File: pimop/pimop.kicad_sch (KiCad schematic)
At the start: 4 parts

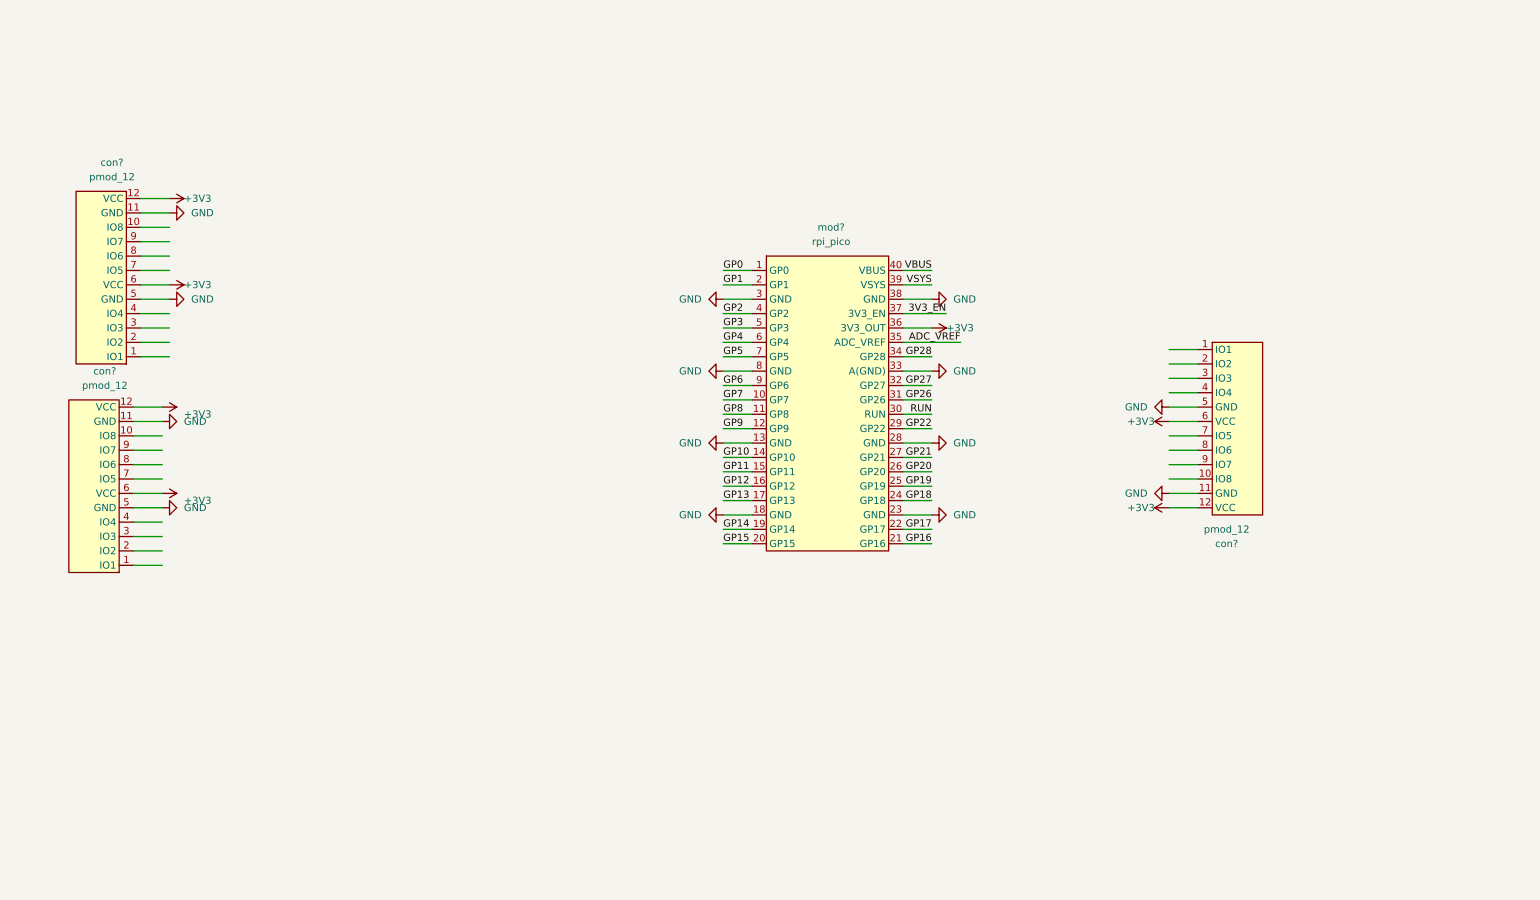
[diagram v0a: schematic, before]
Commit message: schema afgewerkt
schema afgewerkt
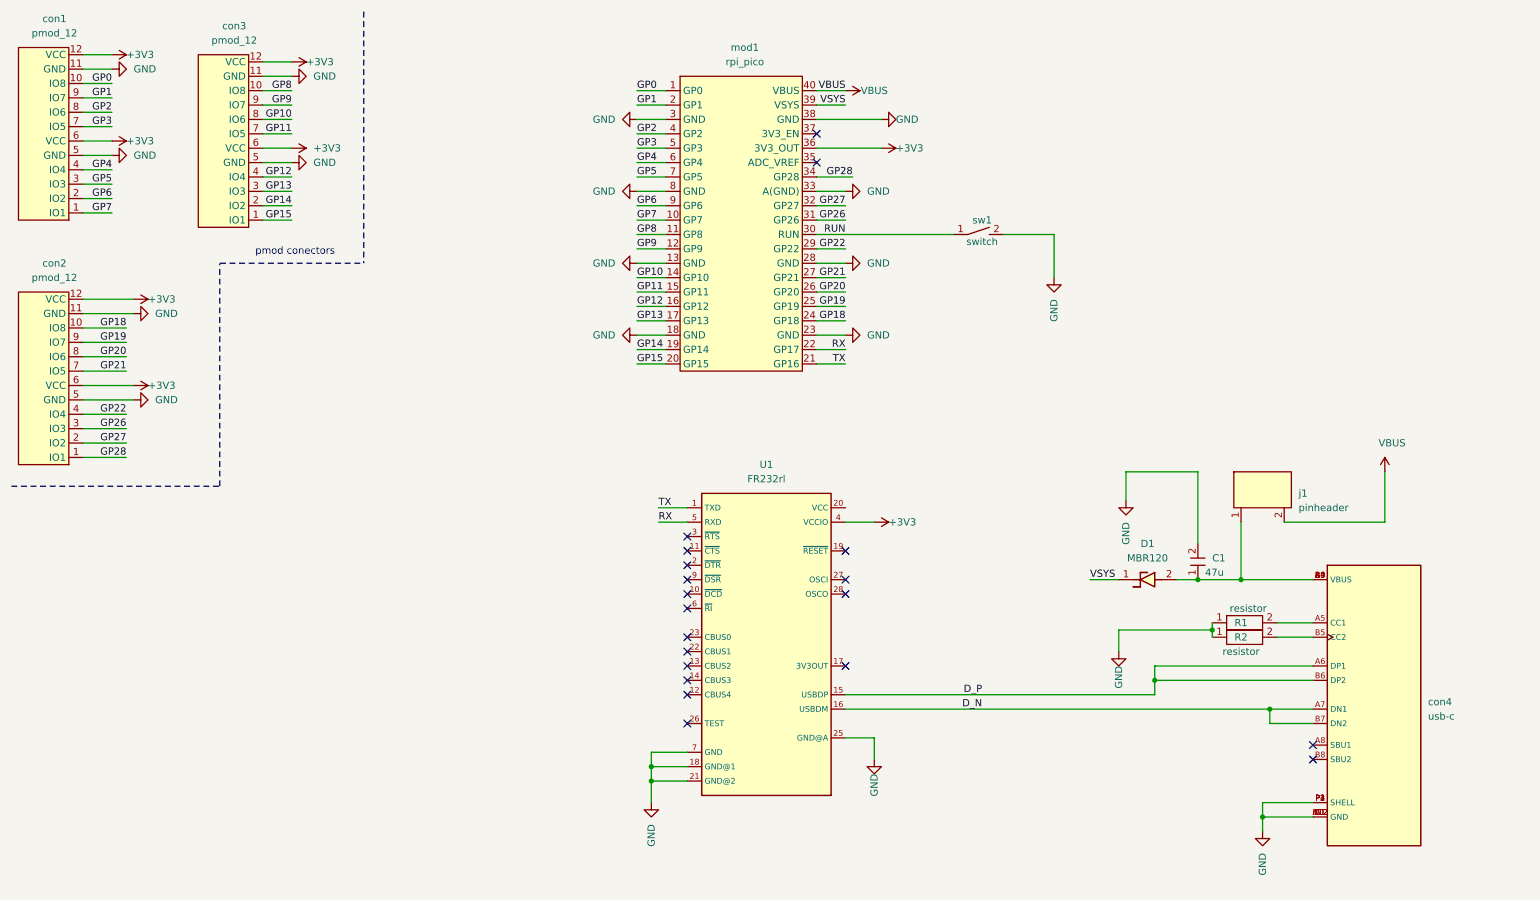
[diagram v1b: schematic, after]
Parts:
- added C1: 47u, vanalles:0603RL, symbol vanalles:capacitor
- added D1: MBR120, halfgeleiders:SOD123, symbol Halfgelijders:MBR120
- added R1, R2: resistor, vanalles:0603RL, symbol vanalles:resistor
- added U1: FR232rl, halfgeleiders:SSOP28-0.65-10.2X5.2MM, symbol Halfgelijders:FR232rl
- added con4: usb-c, connectors_user:GCT_USB4085-GF-A_REVA, symbol connectors:usb-c
- added j1: pinheader, connectors_user:heaer2pin, symbol vanalles:pinheader
- added sw1: switch, vanalles:Alps_SKRK, symbol vanalles:switch
- con1, con2, con3: renamed from con?; footprint (none) -> connectors_user:PMOD12
- mod1: renamed from mod?; footprint (none) -> Module:rpi pico
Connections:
- net +3V3: now also U1.4 (VCCIO)
- net GND: now also C1.2, R1.1, R2.1, U1.18 (GND@1), U1.21 (GND@2), U1.25 (GND@A), U1.7 (GND), con4.A1 (GND), con4.A12 (GND), con4.B1 (GND), con4.B12 (GND), con4.P1 (SHELL), con4.P2 (SHELL), con4.P3 (SHELL), con4.P4 (SHELL), sw1.2
- net GP0: now also con1.10 (IO8)
- net GP1: now also con1.9 (IO7)
- net GP10: now also con3.8 (IO6)
- net GP11: now also con3.7 (IO5)
- net GP12: now also con3.4 (IO4)
- net GP13: now also con3.3 (IO3)
- net GP14: now also con3.2 (IO2)
- net GP15: now also con3.1 (IO1)
- net GP18: now also con2.10 (IO8)
- net GP19: now also con2.9 (IO7)
- net GP2: now also con1.8 (IO6)
- net GP20: now also con2.8 (IO6)
- net GP21: now also con2.7 (IO5)
- net GP22: now also con2.4 (IO4)
- net GP26: now also con2.3 (IO3)
- net GP27: now also con2.2 (IO2)
- net GP28: now also con2.1 (IO1)
- net GP3: now also con1.7 (IO5)
- net GP4: now also con1.4 (IO4)
- net GP5: now also con1.3 (IO3)
- net GP6: now also con1.2 (IO2)
- net GP7: now also con1.1 (IO1)
- net GP8: now also con3.10 (IO8)
- net GP9: now also con3.9 (IO7)
- net RUN: now also sw1.1
- net VBUS: now also j1.2
- net VSYS: now also D1.1
- net 3V3_EN: no longer names the net of mod1.37 (3V3_EN)
- net ADC_VREF: no longer names the net of mod1.35 (ADC_VREF)
- net GP16 renamed TX
- net TX: now also U1.1 (TXD)
- net GP17 renamed RX
- net RX: now also U1.5 (RXD)
- new net: C1.1, D1.2, con4.A4 (VBUS), con4.A9 (VBUS), con4.B4 (VBUS), con4.B9 (VBUS), j1.1
- new net: R1.2, con4.A5 (CC1)
- new net: R2.2, con4.B5 (CC2)
- new net D_N: U1.16 (USBDM), con4.A7 (DN1), con4.B7 (DN2)
- new net D_P: U1.15 (USBDP), con4.A6 (DP1), con4.B6 (DP2)
- no-connect marks 0 -> 20
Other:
- note added: "pmod conectors"
- moved on the sheet: con1, con2, con3, mod1

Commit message: e5yt
45y
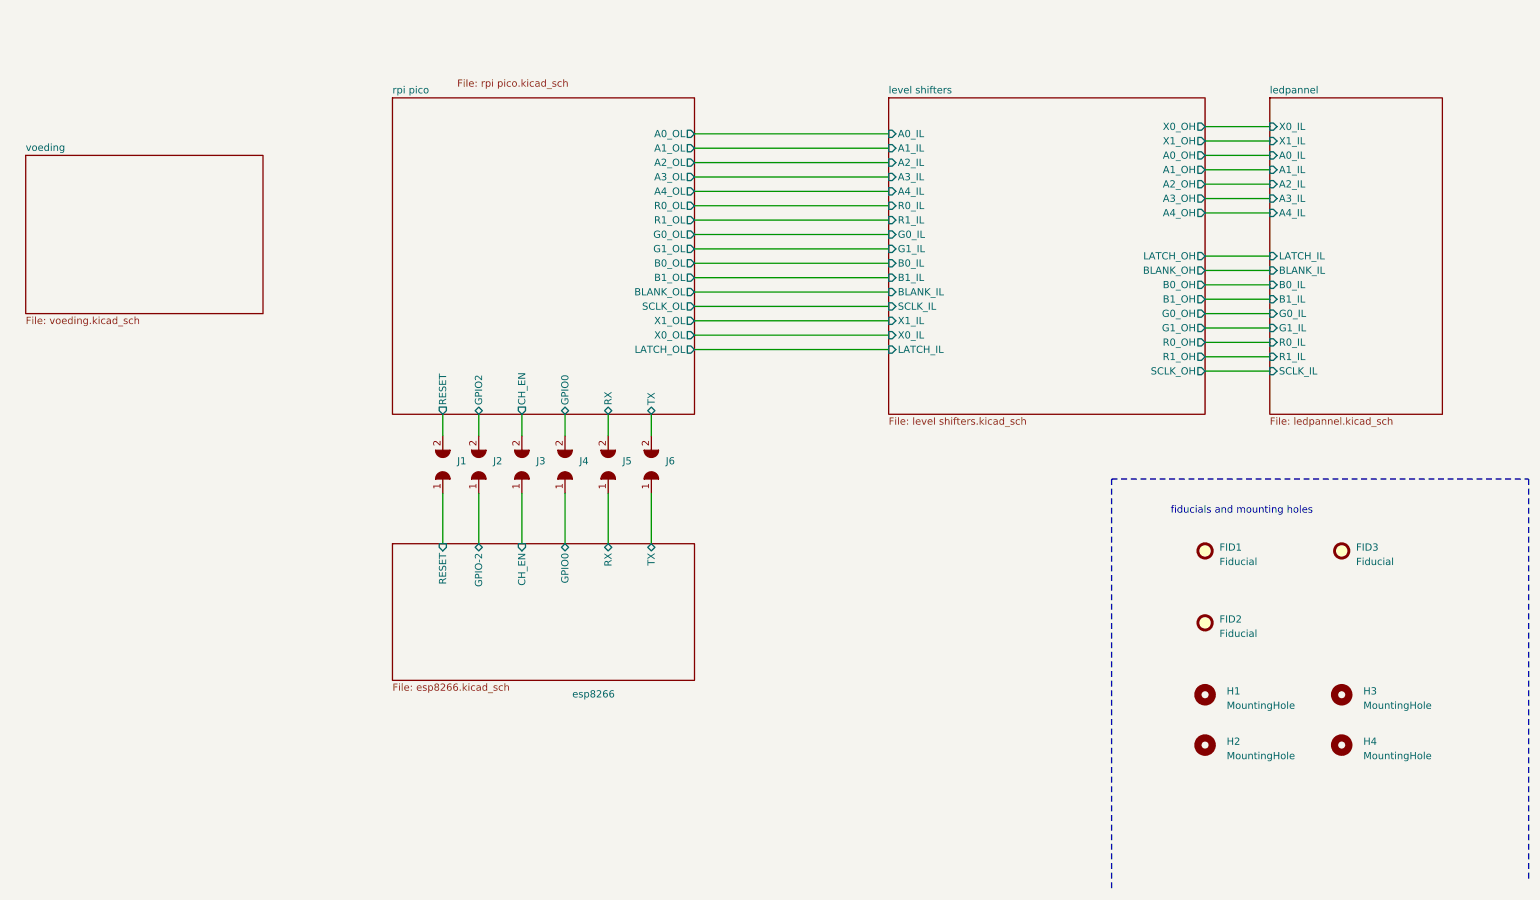
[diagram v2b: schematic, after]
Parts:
- removed C1: 47u, vanalles:0603RL, symbol vanalles:capacitor
- removed D1: MBR120, halfgeleiders:SOD123, symbol Halfgelijders:MBR120
- removed R1, R2: resistor, vanalles:0603RL, symbol vanalles:resistor
- removed U1: FR232rl, halfgeleiders:SSOP28-0.65-10.2X5.2MM, symbol Halfgelijders:FR232rl
- removed con1, con2, con3: pmod_12, connectors_user:PMOD12, symbol connectors:pmod_12
- removed con4: usb-c, connectors_user:GCT_USB4085-GF-A_REVA, symbol connectors:usb-c
- removed j1: pinheader, connectors_user:heaer2pin, symbol vanalles:pinheader
- removed mod1: rpi_pico, Module:rpi pico, symbol modulles:rpi_pico
- removed sw1: switch, vanalles:Alps_SKRK, symbol vanalles:switch
- added FID1, FID2, FID3: Fiducial, vanalles:Fiducial_1.5mm_Mask4.5mm, symbol Mechanical:Fiducial
- added H1, H2, H3, H4: MountingHole, vanalles:MountingHole_2.2mm_M2_Pad, symbol Mechanical:MountingHole
- added J1, J2, J3, J4, J5, J6: solderjumper_2pin, vanalles:SolderJumper-2_P1.3mm_Open_Pad1.0x1.5mm, symbol conectors:solderjumper_2pin
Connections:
- new net esp8266/CH_EN: J3.1
- new net esp8266/GPIO-2: J2.1
- new net esp8266/GPIO0: J4.1
- new net esp8266/RESET: J1.1
- new net esp8266/RX: J5.1
- new net esp8266/TX: J6.1
- new net rpi pico/CH_EN: J3.2
- new net rpi pico/GPIO0: J4.2
- new net rpi pico/GPIO2: J2.2
- new net rpi pico/RESET: J1.2
- new net rpi pico/RX: J5.2
- new net rpi pico/TX: J6.2
- no-connect marks 20 -> 0
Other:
- added sheet esp8266 (esp8266.kicad_sch)
- added sheet ledpannel (ledpannel.kicad_sch)
- added sheet level shifters (level shifters.kicad_sch)
- added sheet rpi pico (rpi pico.kicad_sch)
- added sheet voeding (voeding.kicad_sch)
- note added: "fiducials and mounting holes"
- note removed: "pmod conectors"
